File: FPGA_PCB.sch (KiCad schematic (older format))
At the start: 29 parts, among them J1 Conn_01x01_Male, J10 Conn_Coaxial, J11 Conn_Coaxial, J12 Conn_01x03_Male, J13 Conn_01x03_Male, J14 Conn_01x01_Male, J15 Conn_01x01_Male, J16 73096-2, J17 73096-2, J18 Conn_01x01_Male, J19 Conn_01x01_Male, J2 Conn_01x01_Male, J20 Conn_01x01_Male, J3 73096-2, J4 73096-2, J5 Conn_01x04_Male, J6 Conn_01x04_Male, J7 Conn_01x04_Male, J8 Conn_01x04_Male, J9 Conn_01x04_Male, SW1 SW_Push, U1 CPG08462

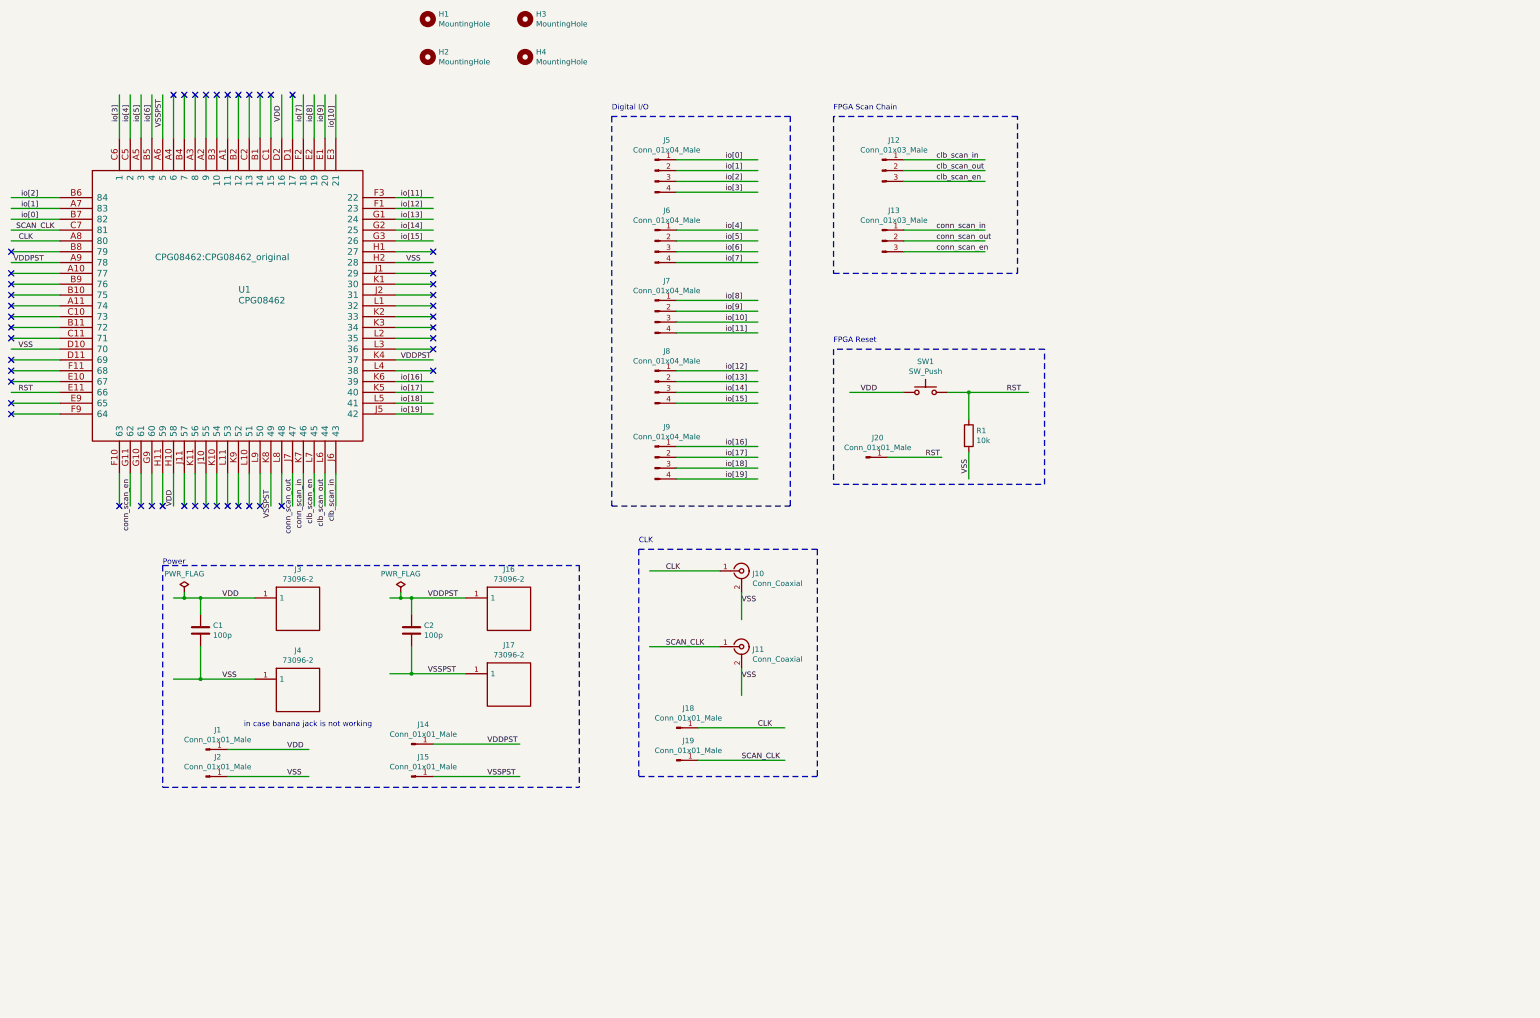
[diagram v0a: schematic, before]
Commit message: ver 2.0
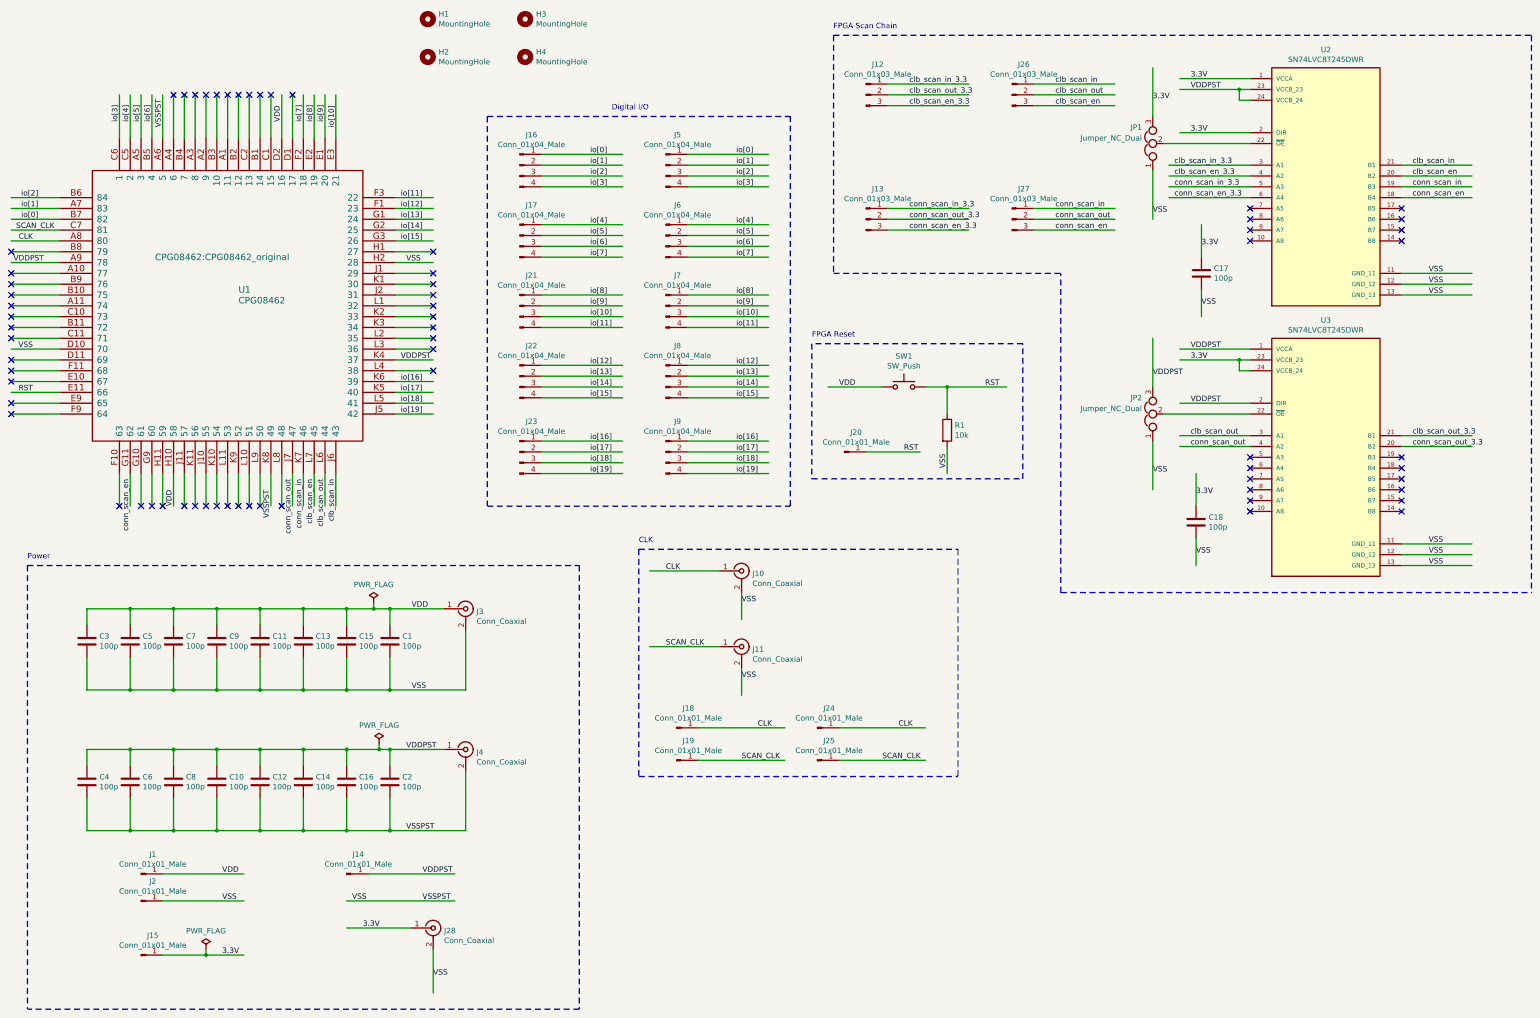
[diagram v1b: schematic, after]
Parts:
- removed J16, J17, J3, J4: 73096-2, 73096-2:73096-2, symbol 73096-2:73096-2
- added C10, C11, C12, C13, C14, C15, C16, C17, C18, C3, C4, C5, C6, C7, C8, C9: 100p, Capacitor_SMD:C_0805_2012Metric_Pad1.15x1.40mm_HandSolder, symbol Device:C
- added J16, J17, J21, J22, J23: Conn_01x04_Male, Connector_PinHeader_2.54mm:PinHeader_1x04_P2.54mm_Vertical, symbol Connector:Conn_01x04_Male
- added J24, J25: Conn_01x01_Male, Connector_PinHeader_2.54mm:PinHeader_1x01_P2.54mm_Vertical, symbol Connector:Conn_01x01_Male
- added J26, J27: Conn_01x03_Male, Connector_PinHeader_2.54mm:PinHeader_1x03_P2.54mm_Vertical, symbol Connector:Conn_01x03_Male
- added J28, J3, J4: Conn_Coaxial, Connector_Coaxial:BNC_TEConnectivity_1478204_Vertical, symbol Connector:Conn_Coaxial
- added JP1, JP2: Jumper_NC_Dual, Connector_PinHeader_2.54mm:PinHeader_1x03_P2.54mm_Vertical, symbol Device:Jumper_NC_Dual
- added U2, U3: SN74LVC8T245DWR, SOIC127P1030X265-24N, symbol SN74LVC8T245DWR:SN74LVC8T245DWR
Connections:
- net labels added: 3.3V, clb_scan_en_3.3, clb_scan_in_3.3, clb_scan_out_3.3, conn_scan_en_3.3, conn_scan_in_3.3, conn_scan_out_3.3
- wire segments 142 -> 269
- no-connect marks 47 -> 67
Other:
- note removed: "in case banana jack is not working"
- moved on the sheet: C1, C2, J1, J12, J13, J14, J2, J20, J5, J6, J7, J8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
